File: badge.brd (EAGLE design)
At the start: 53.8 x 85.3 mm, 33 parts, among them IC1 MCP1703CB, U1 ESP8266, U2 AT25SF041-SOIC8, Y1 26MHz

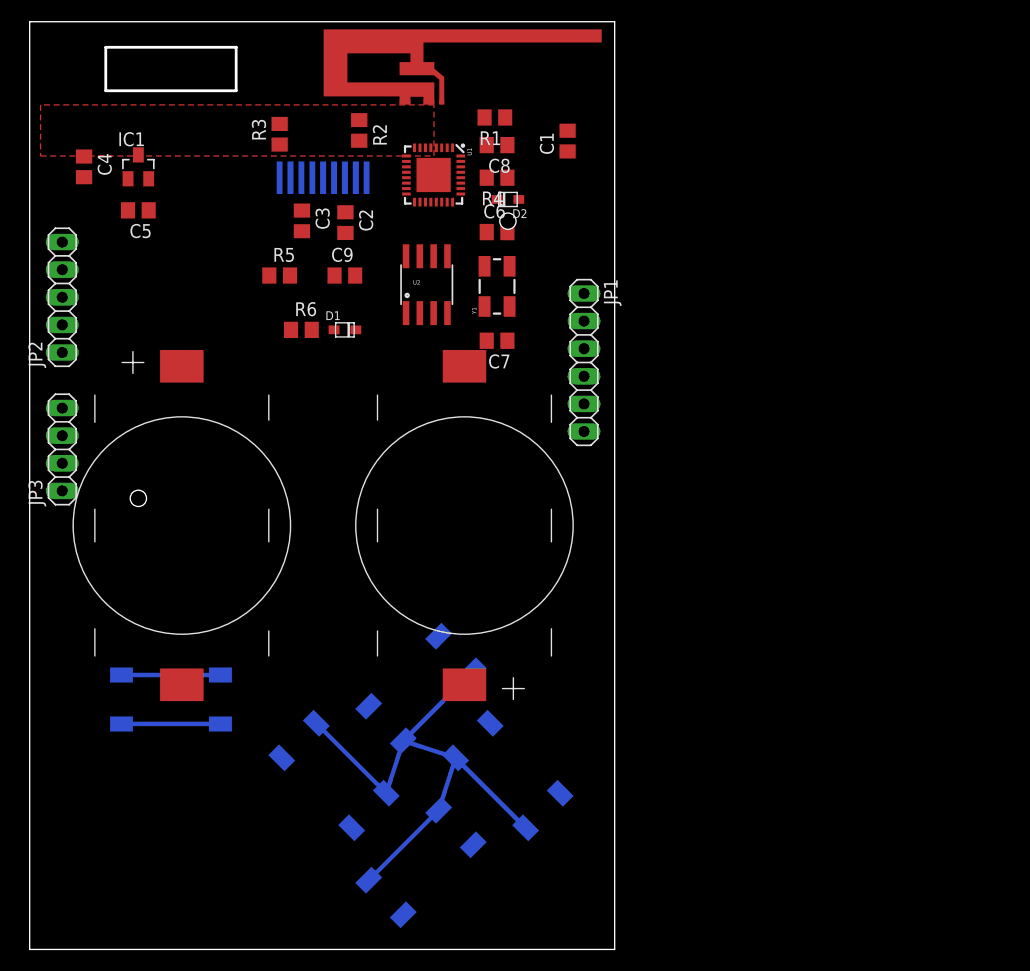
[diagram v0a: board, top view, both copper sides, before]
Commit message: for ys
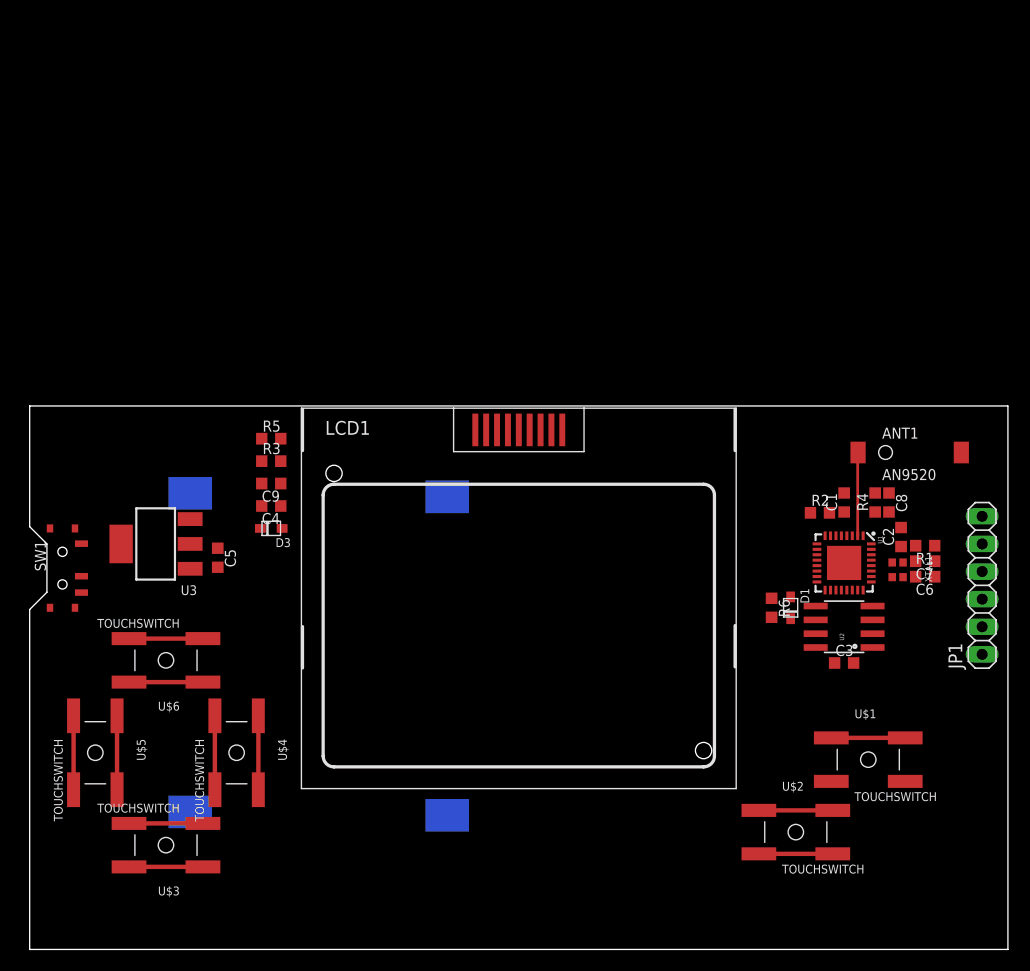
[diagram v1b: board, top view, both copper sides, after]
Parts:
- removed D2: 1N4148, adafruit:SOD-323F
- removed E1: ANTENNATRACE, SparkFun-RF:TRACE_ANTENNA_2.4GHZ_25.7MM
- removed IC1: MCP1703CB, linear:SOT23
- removed JP2: (no value), pinhead:1X05
- removed JP3: (no value), pinhead:1X04
- removed S1, S2, S3, S4, S5: (no value), gm2:TACT-SW-4P-SMD
- removed Y1: 26MHz, SparkFun-FreqCtrl:CRYSTAL-SMD-5X3
- added ANT1: AN9520, badge:AN9520
- added D3: 1N4148, adafruit:SOD-323F
- added SW1: MK12C02, badge:MK12C02
- added U$1, U$2, U$3, U$4, U$5, U$6: TOUCHSWITCH, badge:EVQQWN03W
- added U3: LM317EMP-SOT223, Seeed-OPL-ic:SOT-223
- added XTAL1: 26MHZ, badge:XRCGB_F_P
- C1, C2, C3, C4, C5, C6, C7, C8, C9: device rcl:C0805 -> resistor:C0603K
- R1, R2, R3, R4, R5, R6: device rcl:R0805 -> resistor:R0603W
- moved C3 64.4 mm to (74.9, 26.4), turned to 0 degrees
- moved C2 58.7 mm to (80.2, 37.9), turned to 90 degrees
- moved R1 55.9 mm to (82.4, 37.1)
- moved R2 55.1 mm to (72.7, 40.2), turned to 0 degrees
- moved U1 52.0 mm to (74.9, 35.6)
- moved C6 50.6 mm to (82.4, 34.3), turned to 180 degrees
- moved R6 50.3 mm to (68.3, 31.4), turned to 270 degrees
- moved U2 49.7 mm to (74.9, 29.7), turned to 90 degrees
- moved C8 48.8 mm to (79.1, 41.1), turned to 270 degrees
- moved D1 48.3 mm to (70.0, 31.4), turned to 270 degrees
- moved R4 45.9 mm to (77.8, 41.1), turned to 90 degrees
- moved C7 44.3 mm to (82.4, 35.7)
- moved JP1 42.0 mm to (87.6, 33.5), turned to 90 degrees
- moved C1 41.9 mm to (74.9, 41.1)
- moved C4 35.6 mm to (22.2, 40.8), turned to 180 degrees
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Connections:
- removed net GPIO2: JP3.2, S1.1, S1.2, U1.14
- removed net N$7: C7.1, U1.28, Y1.1
- removed net SPI_CLK: JP2.4, LCD1.2, U1.9
- removed net SPI_CS: JP2.5, S4.1, S4.2, U1.13
- removed net SPI_SI: JP2.3, LCD1.3, U1.12
- removed net SPI_SO: JP2.2, LCD1.4, U1.10
- new net ANT: ANT1.P$1, U1.2
- new net GPIO12/SPI_SO: LCD1.4, U1.10
- new net GPIO13/SPI_SI: LCD1.3, U1.12
- new net GPIO14/SPI_CLK/SCL: LCD1.2, U1.9
- new net GPIO15/SPI_CS: U$3.P$2, U$3.P$3, U$4.P$2, U$4.P$3, U1.13
- new net GPIO16: U1.8
- new net GPIO2/SDA: U$1.P$1, U$1.P$4, U$3.P$1, U$3.P$4, U$5.P$1, U$5.P$4, U1.14
- net 5V: now also D3.A
- net ADC: no longer JP2.1
- net GND: now also C6.1, C7.1, U3.1; no longer C6.2, C7.2, E1.GND, E1.GND2, IC1.1, S1.3, S1.4, S2.3, S2.4, S3.3, S3.4, S4.3, S4.4, S5.3, S5.4
- net GPIO0: now also U$5.P$2, U$5.P$3, U$6.P$2, U$6.P$3; no longer JP3.1, S5.1, S5.2
- net GPIO4: now also U$2.P$1, U$2.P$4, U$4.P$1, U$4.P$4, U$6.P$1, U$6.P$4; no longer JP3.3, S2.1, S2.2
- net GPIO5: now also U$1.P$2, U$1.P$3, U$2.P$2, U$2.P$3; no longer JP3.4, S3.1, S3.2
- net N$1: now also SW1.P$2, U3.3; no longer E1.ANT, U1.2
- net N$5: now also D3.C, SW1.P$1; no longer IC1.3
- net N$6: now also C6.2, U1.27, XTAL1.P$2; no longer D2.C, U1.8
- net N$8: now also C7.2, U1.28, XTAL1.P$4; no longer C6.1, U1.27, Y1.3
- net RESET: no longer D2.A
- net VCC: now also U3.2, U3.TER; no longer IC1.2
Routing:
- net GND: track 60.7 -> 0.00 mm
- net GPIO4: track 0.00 -> 20.4 mm
- net GPIO2/SDA: track 0.00 -> 20.4 mm
- net GPIO15/SPI_CS: track 0.00 -> 13.6 mm
- net ANT: track 0.00 -> 7.69 mm
- net GPIO5: track 0.00 -> 7.41 mm
- net GPIO0: track 9.10 -> 13.6 mm
- removed copper zone on layer 1, net GND
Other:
- board size 53.8 x 85.3 mm -> 90 x 50 mm
